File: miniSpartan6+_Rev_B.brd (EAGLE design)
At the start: 76.2 x 50.8 mm, 95 parts, among them J1 USB-MINIB-5PIN, J2 HDMI-TYPE-A-RECEPTICALFCI1002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, J3 HDMI-TYPE-A-RECEPTICALFCI1002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, J4 P24-1, J5 MICROSD_MOLEX, J6 P24-1, Q1 12MHz, U1 93C46B, U10 SPI_FLASH-SOIC_150_208, U11 PCA9306, U3 ADC088S102CIMT, U4 +3.3V Reg., U5 +1.2V Reg., U6 XC6SLX25-FT256, U7 ASFLMB-32.000MHZ-LC-T, U8 ASFLMB-50.000MHZ-LC-T, U9 SDRAM-16MX16-WINBOND

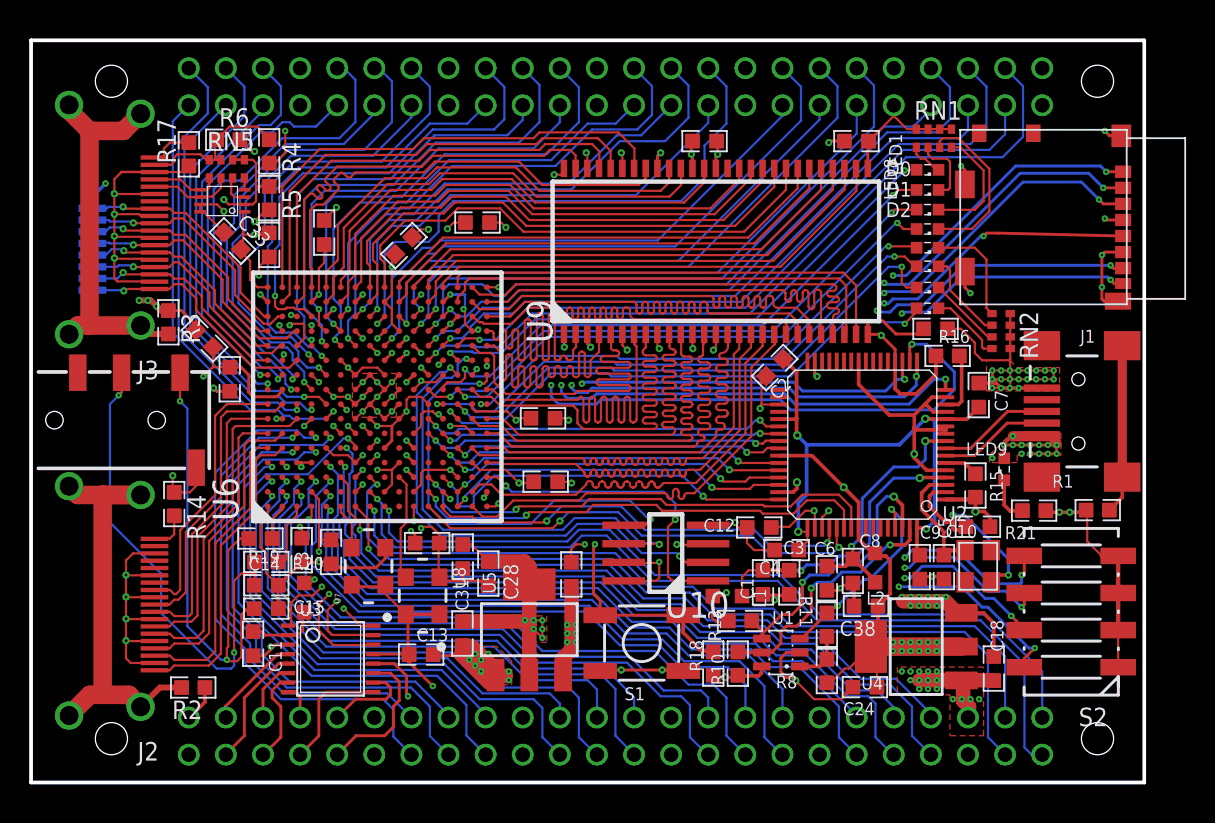
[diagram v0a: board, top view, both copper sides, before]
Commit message: Updating to the current production version
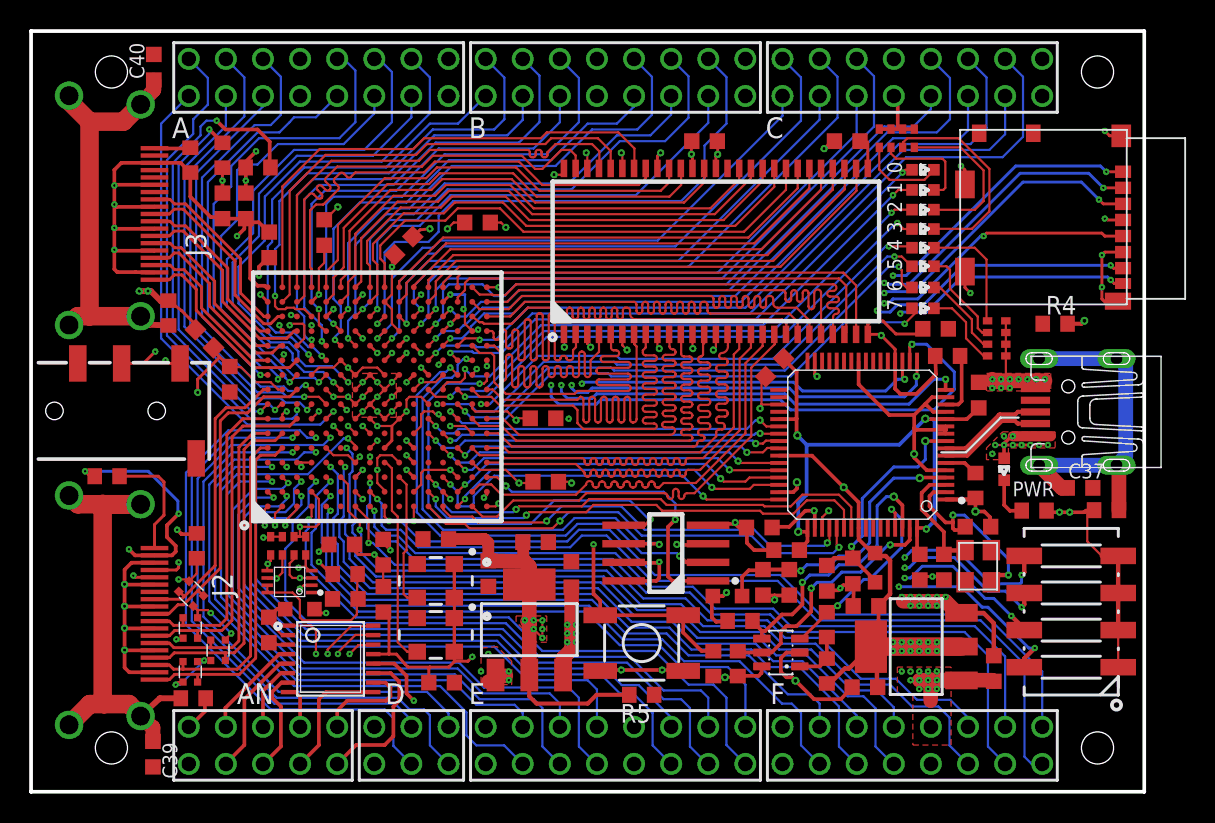
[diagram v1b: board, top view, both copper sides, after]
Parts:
- removed J1: USB-MINIB-5PIN, saanlima:USB-MINIB
- added C37, C39, C40: .1uF, rcl:C0603K
- added R7: 0, rcl:R0603
- added RN8, RN9: 51, resistor-dil:EXB34V
- added X1: MINI-USB-UX60-MB-5S8, con-hirose:UX60-MB-5S8
- C11, C13: value (none) -> 4.7uF
- R4: value 0DNI -> 470
- R5: value 0 -> 470
- RN1, RN2: value (none) -> 1k
- RN3, RN4: value (none) -> 51; device resistor-dil:0603-ARV -> resistor-dil:EXB34V
- RN5: value (none) -> 2k
- U2: value (none) -> FT2232HL
- moved R4 55.1 mm to (70.1, 31.4), turned to 0 degrees
- moved R5 42.5 mm to (41.8, 6.00), turned to 180 degrees
- moved RN4 31.3 mm to (10.9, 7.58), flipped to the top, turned to 0 degrees
- moved R6 30.8 mm to (21.5, 14.3)
- moved C15 27.7 mm to (13.1, 39.5), turned to 270 degrees
- moved RN3 27.2 mm to (12.8, 9.05), flipped to the top, turned to 0 degrees
- moved R20 27.0 mm to (15.5, 42.1)
- moved U11 26.5 mm to (17.7, 13.7)
- moved R19 26.4 mm to (13.1, 42.9), turned to 270 degrees
- moved RN5 26.1 mm to (17.6, 16.2)
- moved C14 26.0 mm to (14.7, 39.5), turned to 270 degrees
- moved C33 25.7 mm to (21.5, 12.6), turned to 180 degrees
- moved C31 10.3 mm to (21.3, 16.3), turned to 0 degrees
- moved C29 9.60 mm to (28.1, 6.83)
- moved C22 9.20 mm to (27.7, 16.7), turned to 180 degrees
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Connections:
- net IO0 renamed PORTA0
- net IO1 renamed PORTA1
- net IO11 renamed PORTA11
- net IO12 renamed PORTB0
- net IO13 renamed PORTB1
- net IO14 renamed PORTB2
- net IO15 renamed PORTB3
- net IO16 renamed PORTB4
- net IO17 renamed PORTB5
- net IO18 renamed PORTB6
- net IO19 renamed PORTB7
- net IO2 renamed PORTA2
- net IO20 renamed PORTB8
- net IO21 renamed PORTB9
- net IO22 renamed PORTB10
- net IO23 renamed PORTB11
- net IO24 renamed PORTC0
- net IO25 renamed PORTC1
- net IO26 renamed PORTC2
- net IO27 renamed PORTC3
- net IO28 renamed PORTC4
- net IO29 renamed PORTC5
- net IO3 renamed PORTA3
- net IO30 renamed PORTC6
- net IO31 renamed PORTC7
- net IO32 renamed PORTC8
- net IO33 renamed PORTC9
- net IO34 renamed PORTC10
- net IO35 renamed PORTC11
- net IO36 renamed PORTD0
- net IO37 renamed PORTD1
- net IO38 renamed PORTD2
- net IO39 renamed PORTD3
- net IO42 renamed PORTE2
- net IO43 renamed PORTE3
- net IO48 renamed PORTE8
- net IO49 renamed PORTE9
- net IO5 renamed PORTA5
- net IO50 renamed PORTE10
- net IO51 renamed PORTE11
- net IO54 renamed PORTF2
- net IO55 renamed PORTF3
- net IO56 renamed PORTF4
- net IO57 renamed PORTF5
- net IO6 renamed PORTA6
- net IO60 renamed PORTF8
- net IO61 renamed PORTF9
- net IO62 renamed PORTF10
- net IO63 renamed PORTF11
- removed net CEC: J3.13
- removed net IO10: U$7.P$7, U6.E10
- removed net IO4: U$7.P$3, U6.A9
- removed net IO40: J4.P$9, U6.D5
- removed net IO41: J6.P$9, U6.A4
- removed net IO44: J4.P$12, U6.A2
- removed net IO45: J6.P$12, U6.B3
- removed net IO46: J4.P$13, U6.B2
- removed net IO47: J6.P$13, U6.C3
- removed net IO52: J4.P$17, U6.E2
- removed net IO53: J6.P$17, U6.E1
- removed net IO58: J4.P$21, U6.F3
- removed net IO59: J6.P$21, U6.G1
- removed net IO7: U$8.P$5, U6.C9
- removed net IO8: U$7.P$6, U6.C10
- removed net IO9: U$8.P$6, U6.D9
- removed net N$22: J1.MTN1, J1.MTN3, R1.2
- removed net N$35: R5.2, RN3.1, RN3.2, RN3.3, RN3.4, RN4.1, RN4.2, RN4.3, RN4.4
- new net N$13: C37.1, R1.2, X1.M1, X1.M2, X1.M3, X1.M4
- new net N$8: R7.2, RN3.1, RN3.3, RN4.1, RN4.3, RN8.1, RN8.3, RN9.1, RN9.3
- new net PORTA10: U$7.P$7, U6.F10
- new net PORTA4: U$7.P$3, U6.D9
- new net PORTA7: U$8.P$5, U6.C10
- new net PORTA8: U$7.P$6, U6.E10
- new net PORTA9: U$8.P$6, U6.F9
- new net PORTE0: J4.P$10, U6.D5
- new net PORTE1: J6.P$10, U6.A4
- new net PORTE4: J4.P$12, U6.B3
- new net PORTE5: J6.P$12, U6.A2
- new net PORTE6: J4.P$14, U6.B2
- new net PORTE7: J6.P$14, U6.C3
- new net PORTF0: J4.P$18, U6.E2
- new net PORTF1: J6.P$18, U6.E1
- new net PORTF6: J4.P$22, U6.F3
- new net PORTF7: J6.P$22, U6.G1
- net 1V2: now also R5.2
- net 3V3: now also J4.P$13, J4.P$21, J6.P$17, J6.P$9, R4.2, R7.1; no longer J4.P$14, J4.P$22, J6.P$10, J6.P$18, R5.1
- net 5V0: now also X1.1; no longer J1.VBUS, R4.2
- net AD_DIN: now also U6.H4; no longer U6.G6
- net AD_SCLK: now also U6.G6; no longer U6.H4
- net AUDIO1: now also U6.B8; no longer U6.B1
- net AUDIO2: now also U6.A8; no longer U6.C1
- net A_TMDS0_N: no longer RN4.7
- net A_TMDS0_P: no longer RN4.8
- net A_TMDS1_N: no longer RN3.5
- net A_TMDS1_P: no longer RN3.6
- net A_TMDS2_N: no longer RN3.7
- net A_TMDS2_P: no longer RN3.8
- net A_TMDS_CLK_N: no longer RN4.5
- net A_TMDS_CLK_P: no longer RN4.6
- net DDC_SCL: now also J2.15; no longer J3.15
- net DDC_SDA: now also J2.16; no longer J3.16
- net FPGA-CLK-2: now also U6.J4; no longer U6.F1
- net FPGA_SCL: now also U6.C1
- net FPGA_SDA: now also U6.B1
- net GND: now also C37.2, C39.2, C40.2, J4.P$17, J4.P$9, J6.P$13, J6.P$21, R4.1, R5.1, X1.5; no longer J1.GND, J4.P$10, J4.P$18, J6.P$14, J6.P$22, R14.1
- net N$10: now also X1.2; no longer J1.D-
- net N$14: now also X1.3; no longer J1.D+
- net N$24: now also JP5.TIP; no longer JP5.RING1
- net N$25: now also JP5.RING1; no longer JP5.TIP
- net N$34: now also C39.1
- net N$36: now also C40.1
- net TMDS0_N: now also RN8.4
- net TMDS0_P: now also RN8.2
- net TMDS1_N: now also RN3.4
- net TMDS1_P: now also RN3.2
- net TMDS2_N: now also RN4.4
- net TMDS2_P: now also RN4.2
- net TMDS_CLK_N: now also RN9.4, U6.A9; no longer U6.A8
- net TMDS_CLK_P: now also RN9.2, U6.C9; no longer U6.B8
- net TX_HDMI_5V: now also J2.18, R14.1; no longer J3.18, R4.1
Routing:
- net PORTF6: track 0.00 -> 54.4 mm, vias 0 -> 1
- net IO58: track 51.7 -> 0.00 mm, vias 1 -> 0
- net PORTF7: track 0.00 -> 49.5 mm, vias 0 -> 1
- net IO59: track 46.8 -> 0.00 mm, vias 1 -> 0
- net PORTF0: track 0.00 -> 46.5 mm, vias 0 -> 1
- net IO52: track 44.4 -> 0.00 mm, vias 1 -> 0
- net PORTE6: track 0.00 -> 44.3 mm, vias 0 -> 1
- net PORTE0: track 0.00 -> 43.6 mm, vias 0 -> 1
- net PORTF1: track 0.00 -> 43.3 mm, vias 0 -> 1
- net PORTE7: track 0.00 -> 43.2 mm, vias 0 -> 1
- net PORTE4: track 0.00 -> 42.5 mm, vias 0 -> 1
- net GND: track 290.2 -> 248.9 mm, vias 114 -> 91
- net IO53: track 40.8 -> 0.00 mm, vias 1 -> 0
- net 5V0: track 157.9 -> 119.4 mm, vias 26 -> 21
- net PORTE5: track 0.00 -> 38.5 mm, vias 0 -> 1
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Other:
- board size 76.2 x 50.8 mm -> 76.2 x 52.1 mm
- board text added: "0"
- board text added: "2"
- board text added: "3"
- board text added: "4"
- board text added: "5"
- board text added: "6"
- board text added: "7"
- board text added: "A"
- board text added: "AN"
- board text added: "B"
- board text added: "C"
- board text added: "D"
- board text added: "E"
- board text added: "F"
- board text added: "J3"
- board text added: "PWR"
- board text removed: "3V3"
- board text removed: "5V0"
- board text removed: "A0"
- board text removed: "A1"
- board text removed: "A2"
- board text removed: "A3"
- board text removed: "A4"
- board text removed: "A5"
- board text removed: "A6"
- board text removed: "A7"
- board text removed: "A8"
- board text removed: "AN0"
- board text removed: "AN1"
- board text removed: "AN2"
- board text removed: "AN3"
- board text removed: "AN4"
- board text removed: "AN5"
- board text removed: "AN6"
- board text removed: "AN7"
- board text removed: "B0"
- board text removed: "B1"
- board text removed: "B2"
- board text removed: "B3"
- board text removed: "B4"
- board text removed: "B5"
- board text removed: "B6"
- board text removed: "B7"
- board text removed: "B8"
- board text removed: "C0"
- board text removed: "C1"
- board text removed: "C2"
- board text removed: "C3"
- board text removed: "C4"
- board text removed: "C5"
- board text removed: "C6"
- board text removed: "C7"
- board text removed: "C8"
- board text removed: "D0"
- board text removed: "D1"
- board text removed: "D2"
- board text removed: "D3"
- board text removed: "D4"
- board text removed: "D5"
- board text removed: "D6"
- board text removed: "D7"
- board text removed: "D8"
- board text removed: "GND"
- board text removed: "J1"
- board text removed: "JTAG"
- board text removed: "LED1"
- board text removed: "LED2"
- board text removed: "LED3"
- board text removed: "LED4"
- board text removed: "LED5"
- board text removed: "LED6"
- board text removed: "LED7"
- board text removed: "LED8"
- board text removed: "PB0"
- board text removed: "PB1"
- board text removed: "PB2"
- board text removed: "PB3"
- board text removed: "PB4"
- board text removed: "PB5"
- board text removed: "PB6"
- board text removed: "PB7"
- board text removed: "PC0"
- board text removed: "PC1"
- board text removed: "PC2"
- board text removed: "PC3"
- board text removed: "PC4"
- board text removed: "PC5"
- board text removed: "PC6"
- board text removed: "PC7"
- board text removed: "PD0"
- board text removed: "PD1"
- board text removed: "PD2"
- board text removed: "PD3"
- board text removed: "PD4"
- board text removed: "PD5"
- board text removed: "PD6"
- board text removed: "PD7"
- board text removed: "RX"
- board text removed: "SW1"
- board text removed: "TX"
